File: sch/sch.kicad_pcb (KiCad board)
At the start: 2 copper layers, 20 parts, among them J1 swd, J2 JOY_CON, J3 USB, U1 STM32F103C8Tx_usb, U2 L78L33_SOT89, Y1 8M

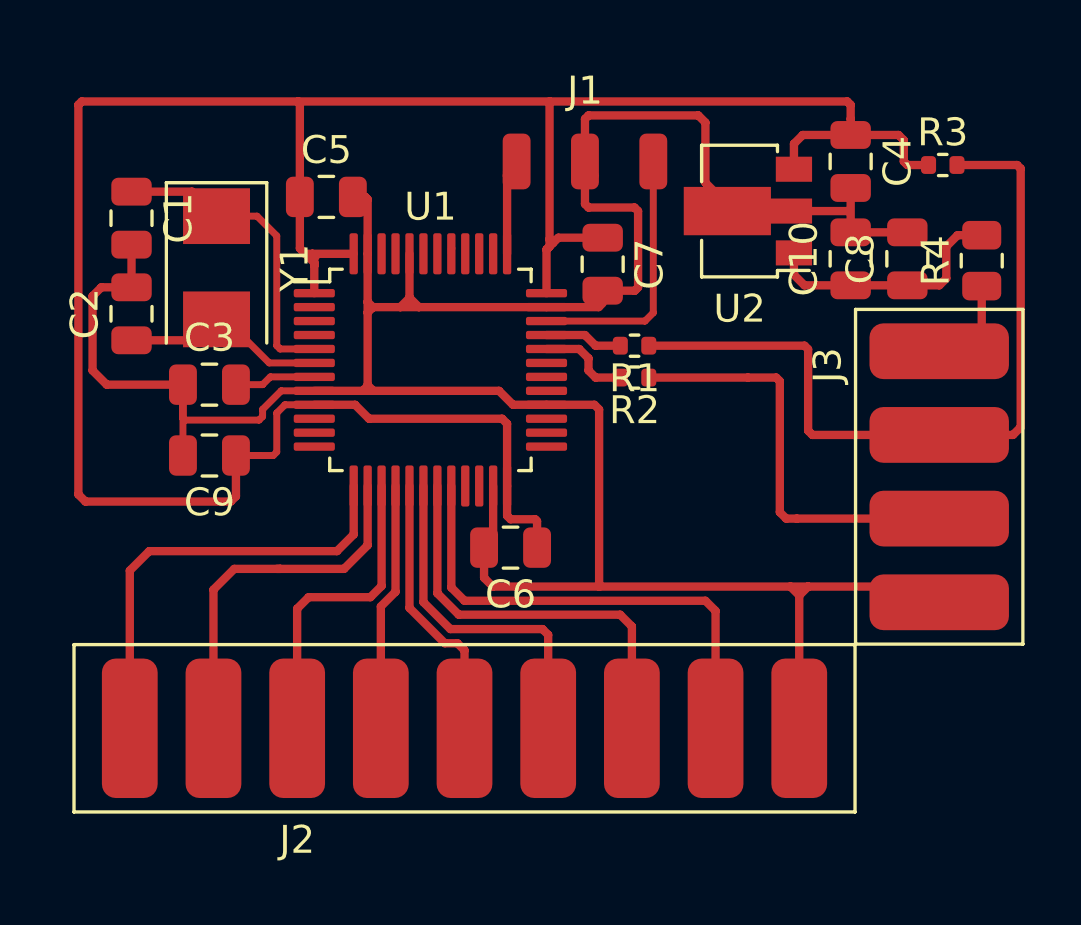
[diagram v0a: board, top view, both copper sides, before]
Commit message: err in pcb
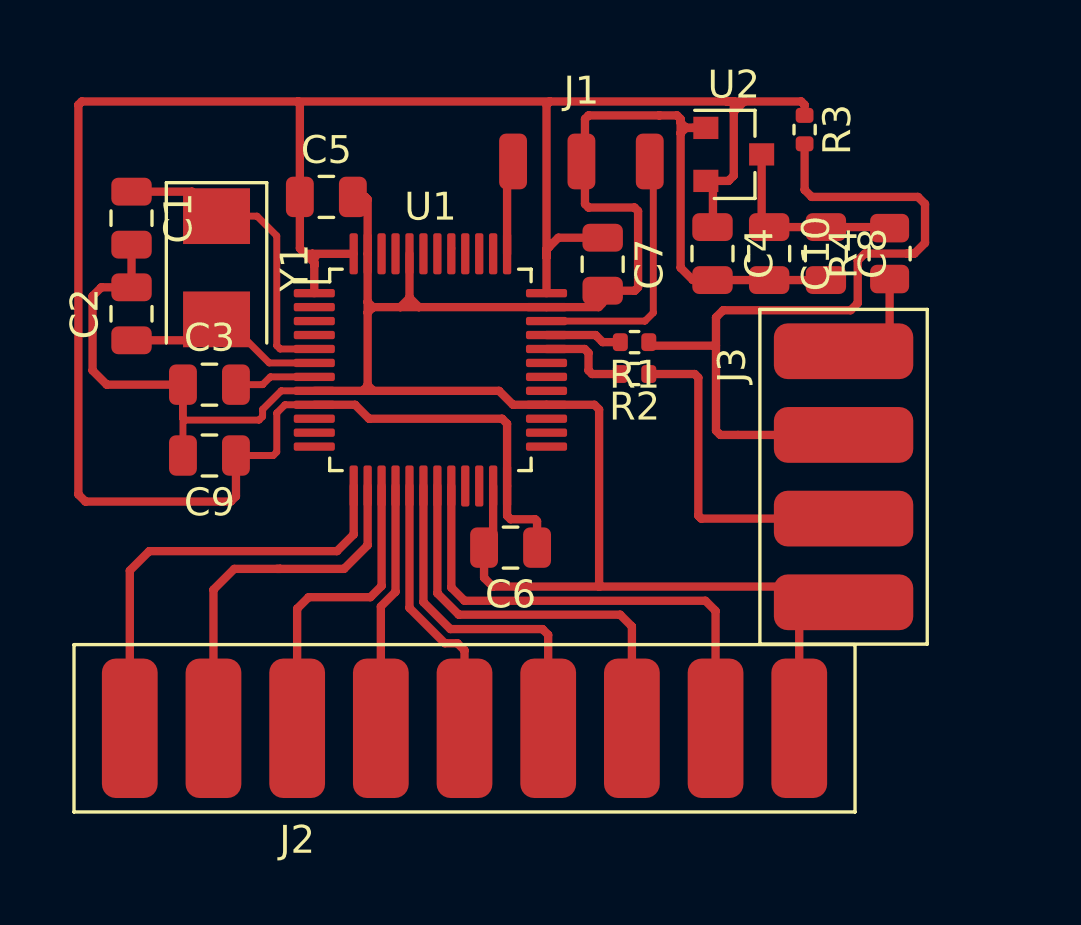
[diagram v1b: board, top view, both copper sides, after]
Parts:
- U2: value L78L33_SOT89 -> XC6206-33; footprint Package_TO_SOT_SMD:SOT-89-3 -> Package_TO_SOT_SMD:SOT-23
- moved C4 5.95 mm to (44.5, 22.6)
- moved R3 5.11 mm to (47.8, 18.2), turned to 270 degrees
- moved J3 3.43 mm to (49.1, 30.6)
- moved R4 3.31 mm to (50.8, 22.6)
- moved C10 2.93 mm to (46.5, 22.6), turned to 270 degrees
- moved C8 2.93 mm to (48.5, 22.6), turned to 270 degrees
- moved U2 2.09 mm to (45.2, 19.1), turned to 0 degrees
- moved J1 0.13 mm to (39.8, 19.3)
- moved R1 0.13 mm to (41.7, 25.8)
- moved R2 0.13 mm to (41.7, 26.9)
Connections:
- U2 pad 1: Net-(C10-Pad1) -> GND
- U2 pad 2: GND -> +3V3
- U2 pad 3: +3V3 -> Net-(C10-Pad1)
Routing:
- net GND: track 115.6 -> 105.3 mm
- net Net-(J3-Pad3): track 15.3 -> 12.0 mm
- net +3V3: track 97.7 -> 95.1 mm
- net Net-(C10-Pad1): track 9.09 -> 6.80 mm
